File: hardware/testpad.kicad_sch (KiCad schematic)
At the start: 14 parts, among them U2 ESP32-C6-WROOM-1, U3 TPS62840YBGR

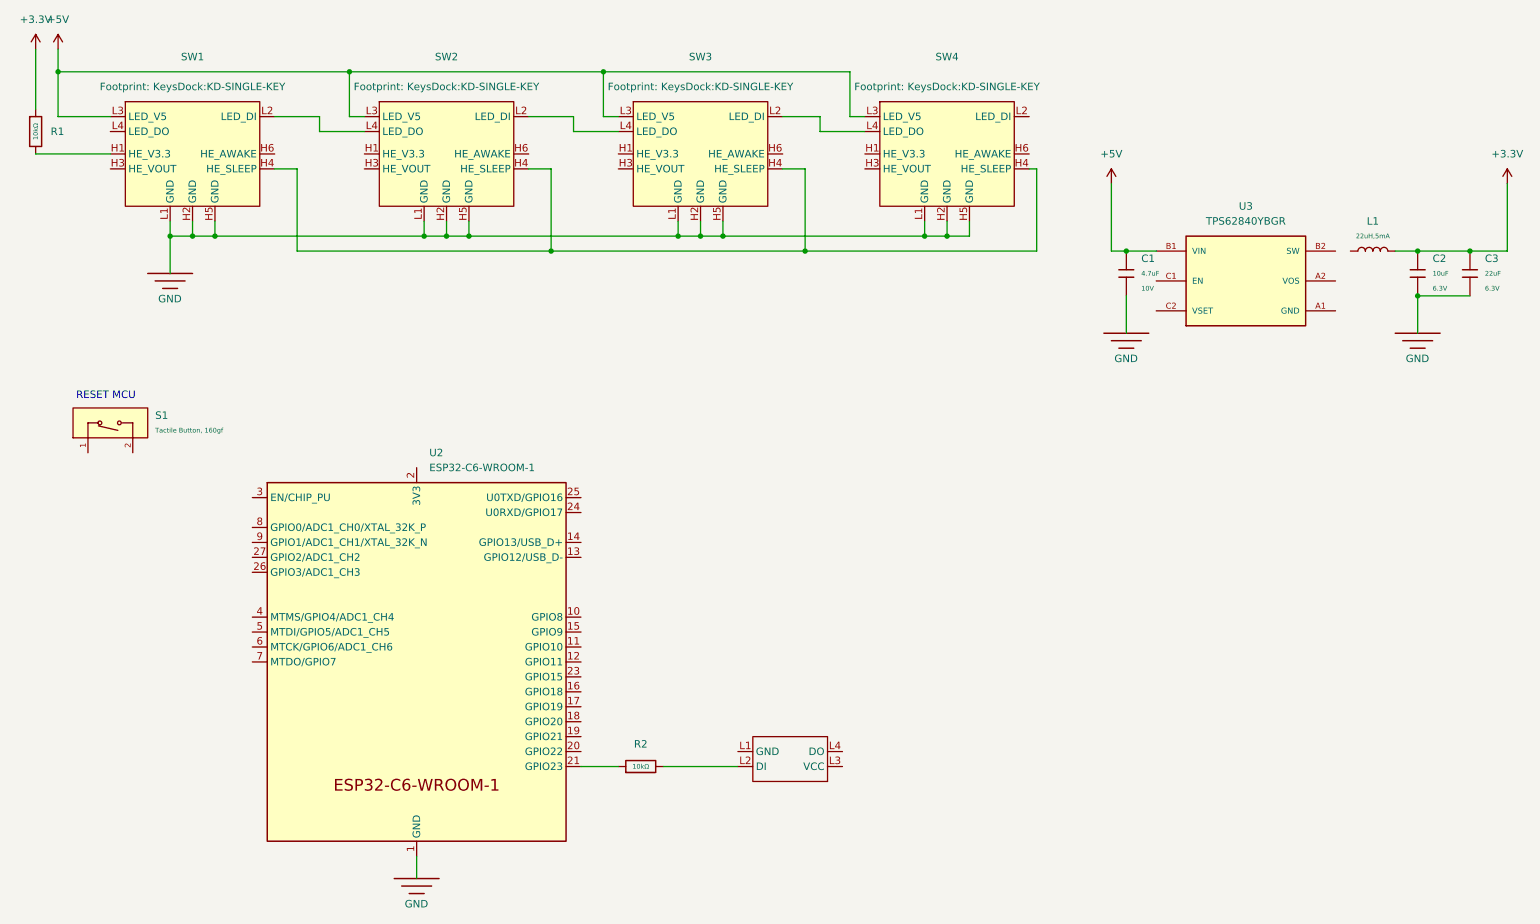
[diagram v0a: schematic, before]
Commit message: :construction: sync components
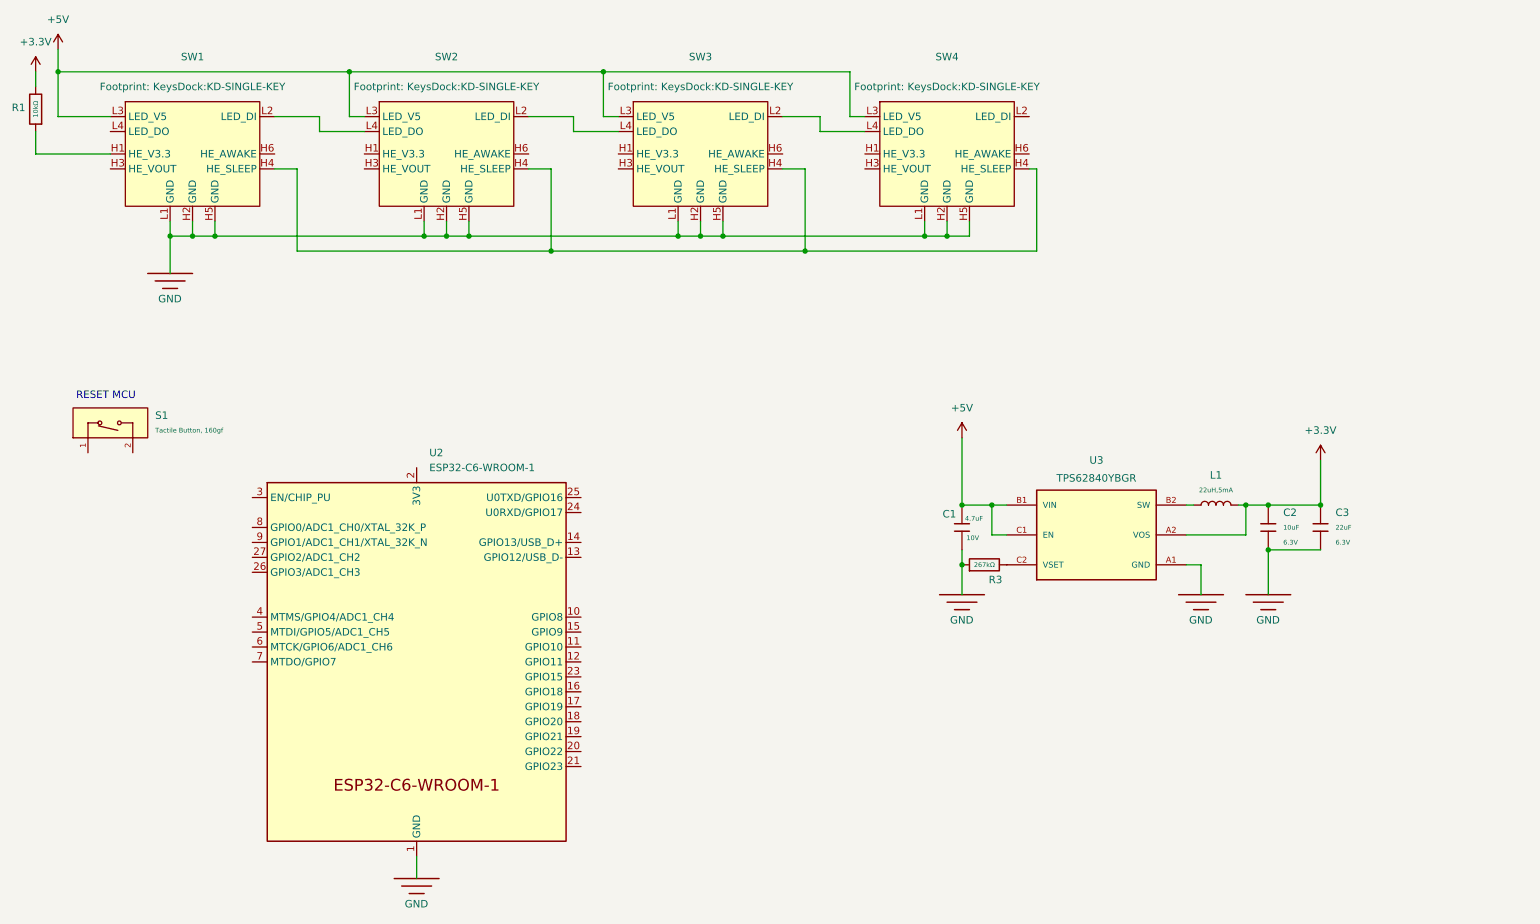
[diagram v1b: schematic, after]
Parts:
- removed D1: LED, symbol components:XL-6028RGBW-WS2812B
- removed L1: 22uH,5mA, PCM_JLCPCB:L_0805, symbol components:22uH,5mA
- removed R2: 10kΩ, KeysDock:R_0402, symbol components:0402,10kΩ
- added L1: 22uH,5mA, KeysDock:IND-SMD_L2.5-W2.0_MHCHL2520, symbol components:FTC252012S2R2MBCA
- added R3: 267kΩ, KeysDock:R_0402, symbol components:0402,267kΩ
- U3: footprint TPS62840YBGR:BGA6N40P3X2_146X96X50N -> KeysDock:BGA6N40P3X2_146X96X50N
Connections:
- net +3.3V: now also R1.2, U3.A2 (VOS), L1.2; no longer R1.1
- net +5V: now also U3.C1 (EN)
- net GND: now also U3.A1 (GND), R3.1
- net at SW1.H1 (HE_V3.3): now also R1.1; no longer R1.2
- net at U3.B2 (SW): now also L1.1
- net at U3.C2 (VSET): now also R3.2
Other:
- moved on the sheet: C1, C2, C3, U3
